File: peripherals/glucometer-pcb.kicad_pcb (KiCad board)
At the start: 2 copper layers, 43.9 x 66.9 mm, 15 parts, among them U1 ESP32_DevKit_V1_DOIT

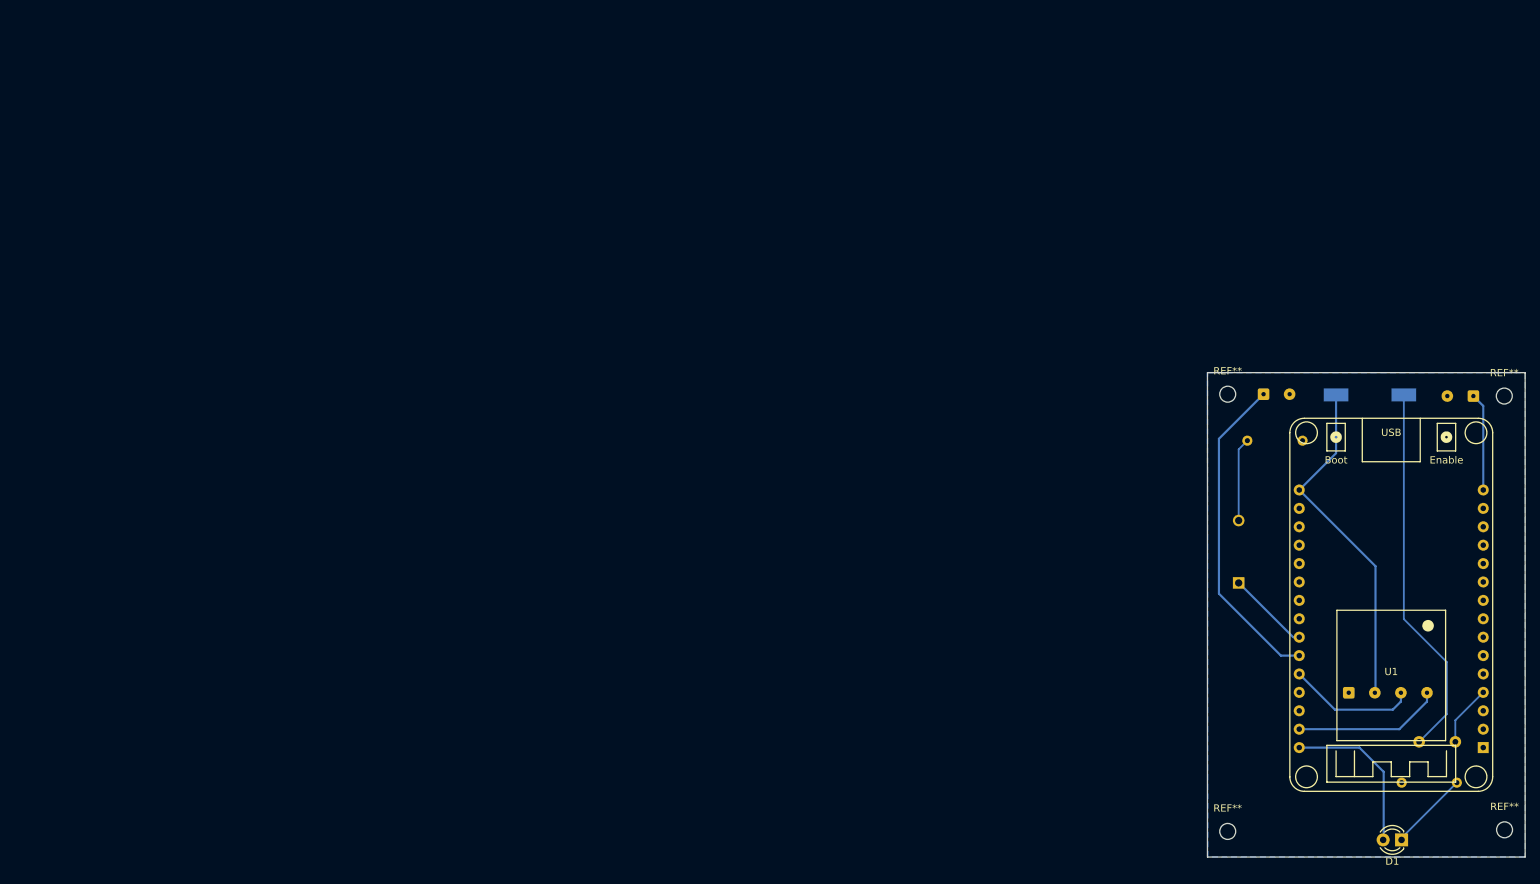
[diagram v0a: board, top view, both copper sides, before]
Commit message: updated pcbs
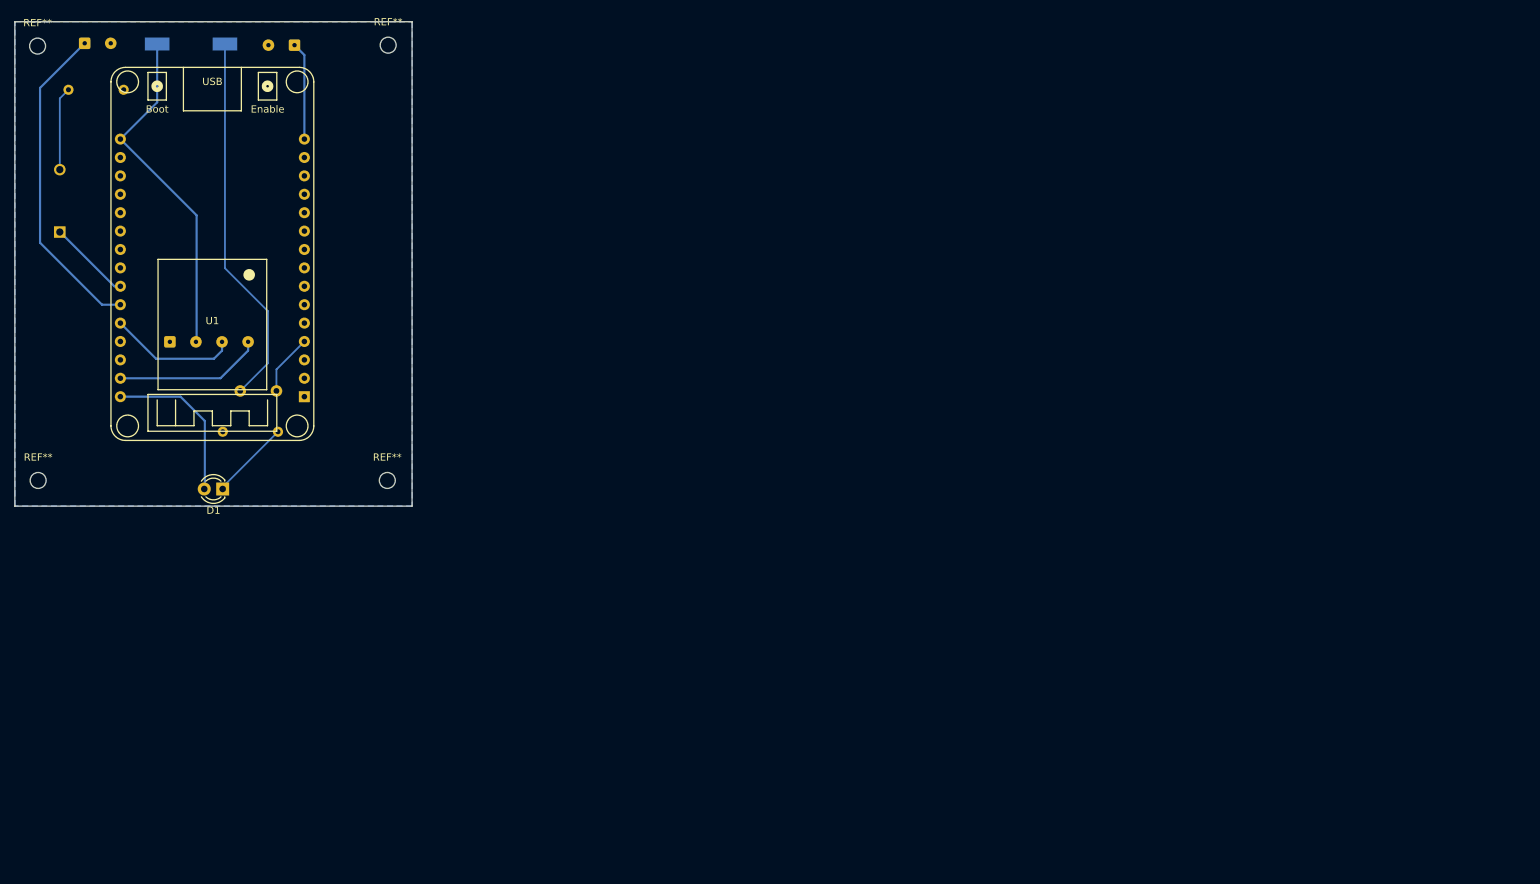
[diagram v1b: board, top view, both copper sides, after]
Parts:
- moved REF** 171.2 mm to (21.5, 82.5)
- moved REF** 171.2 mm to (21.4, 22.5)
- moved INTERRUPT_GPIO1 169.8 mm to (27.9, 22.2)
- moved R1 169.8 mm to (25.7, 28.6)
- moved SIGNAL_IN1 169.8 mm to (47.3, 22.3)
- moved 100nF1 169.8 mm to (49.4, 70.1)
- moved 3V3_OUT1 169.8 mm to (37.9, 22.3)
- moved BATTERY1 169.8 mm to (56.9, 22.4)
- moved BZ1 169.8 mm to (24.5, 47.8)
- moved D1 169.8 mm to (47.0, 83.7)
- moved OLED_PINS1 169.8 mm to (49.8, 63.4)
- moved R2 169.8 mm to (54.6, 75.8)
- moved U1 169.8 mm to (45.5, 70.9)
- moved REF** 161.6 mm to (69.7, 82.5)
- moved REF** 161.5 mm to (69.8, 22.4)
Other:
- board size 43.9 x 66.9 mm -> 54.8 x 66.9 mm
